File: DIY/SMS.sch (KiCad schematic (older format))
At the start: 7 parts, among them J1 Atari_SEGA_DE9, J2 Atari_SEGA_DE9, J3 DB25_Male, U1 74AHCT125N, U2 74AHCT125N, U3 74AHCT125N, U4 74AHCT125N

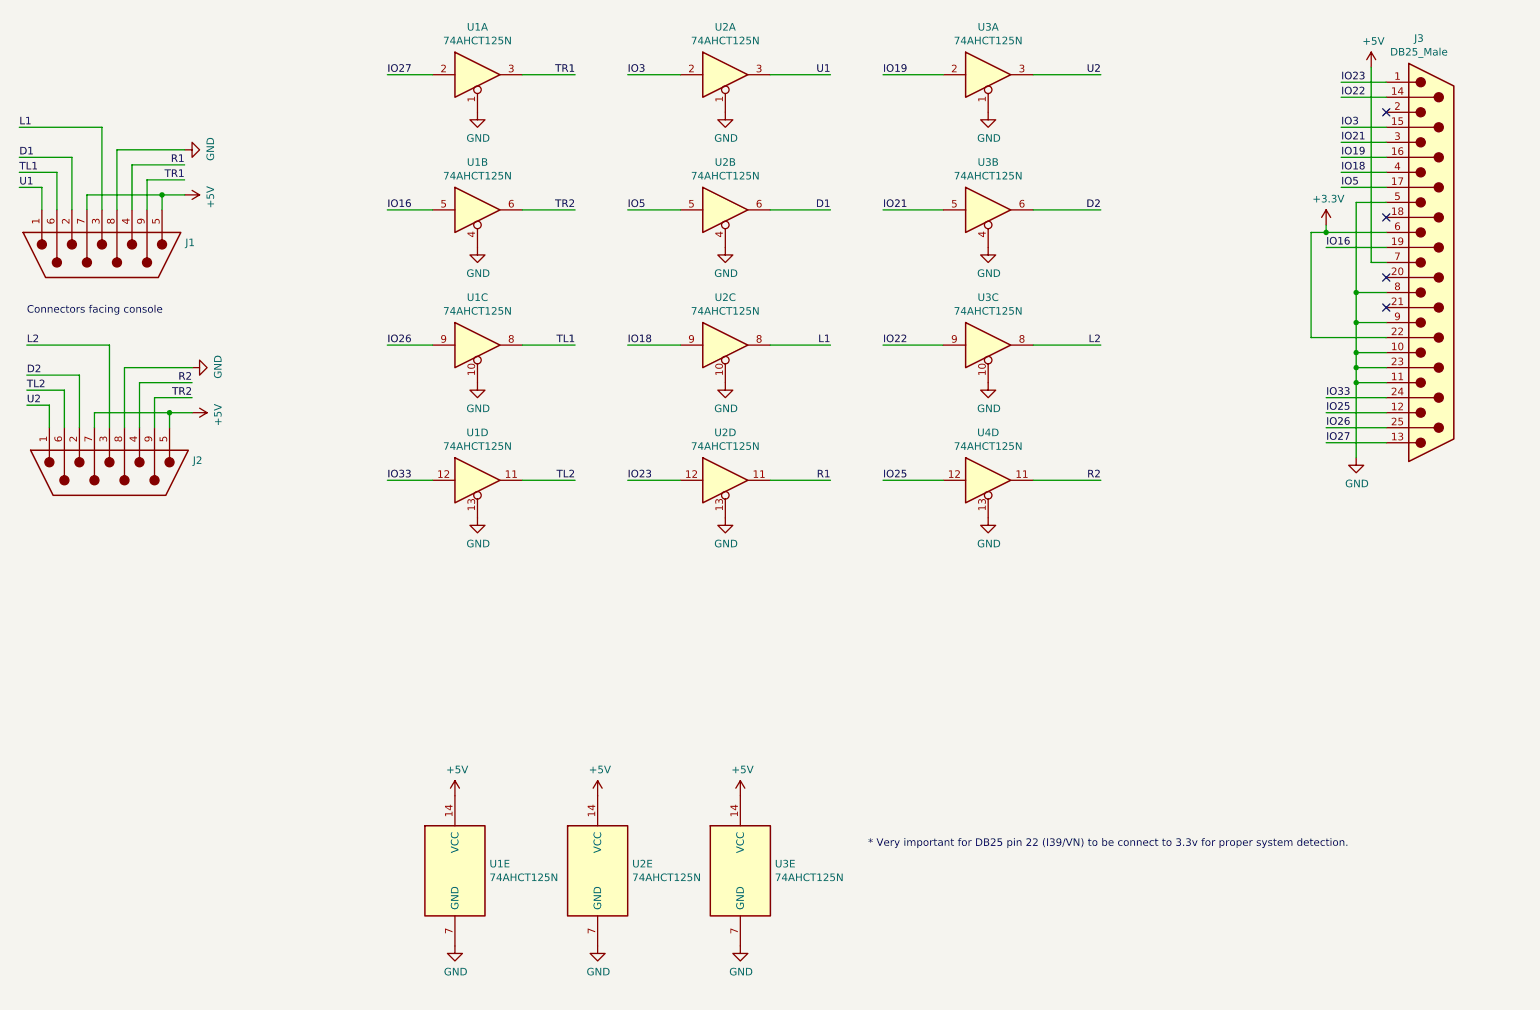
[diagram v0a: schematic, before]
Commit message: [DIY] Add 7800 2 btns adapter
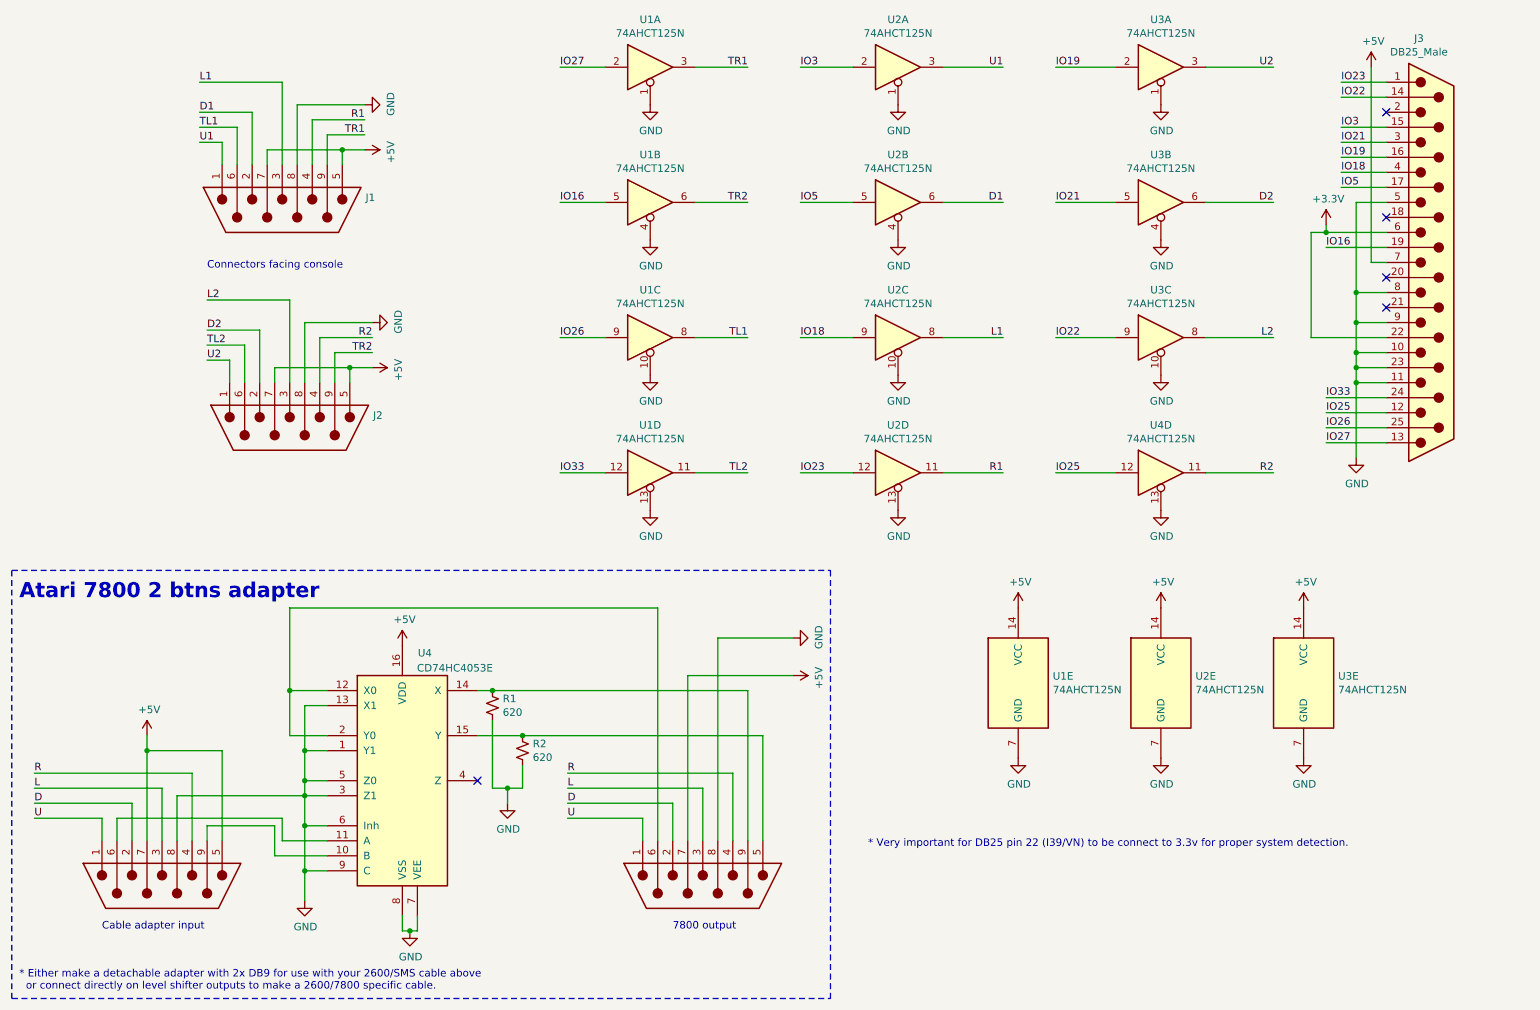
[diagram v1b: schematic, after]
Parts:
- added J? (x2): Atari_SEGA_DE9, symbol Connector_Gaming:Atari_SEGA_DE9
- added R1, R2: 620, symbol Device:R_Small_US
- added unit 1 of U4
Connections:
- net +5V: now also J?.5, J?.7, J?.7, U4.16 (VDD)
- net GND: now also J?.8, J?.8, R1.2, R2.2, U4.1 (Y1), U4.13 (X1), U4.3 (Z1), U4.5 (Z0), U4.6 (Inh), U4.7 (VEE), U4.8 (VSS), U4.9 (C)
- new net: J?.9, U4.10 (B)
- new net: J?.6, U4.11 (A)
- new net: J?.6, U4.12 (X0), U4.2 (Y0)
- new net: J?.9, R1.1, U4.14 (X)
- new net: J?.5, R2.1, U4.15 (Y)
- new net D: J?.2, J?.2
- new net L: J?.3, J?.3
- new net R: J?.4, J?.4
- new net U: J?.1, J?.1
- no-connect marks 4 -> 5
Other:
- note added: "* Either make a detachable adapter with 2x DB9 for use with your 2600/SMS cable above\n or connect directly on level shifter outputs to make a 2600/7800 specific cable."
- note added: "7800 output"
- note added: "Atari 7800 2 btns adapter"
- note added: "Cable adapter input"
- moved on the sheet: J1, J2, U1A, U1B, U1C, U1D, U1E, U2A, U2B, U2C, U2D, U2E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
